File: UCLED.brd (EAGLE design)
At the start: 100 x 20 mm, 35 parts, among them CON1 CON-4P-TABS-JST_GH-RA, CON2 CON-4P-TABS-JST_GH-RA, CON3 PINHEAD_1X06-2, IC1 TJA1051, IC2 STM32F042F4PX, IC3 AP2127-3.3, J1 CONNECTION, J2 CONNECTION

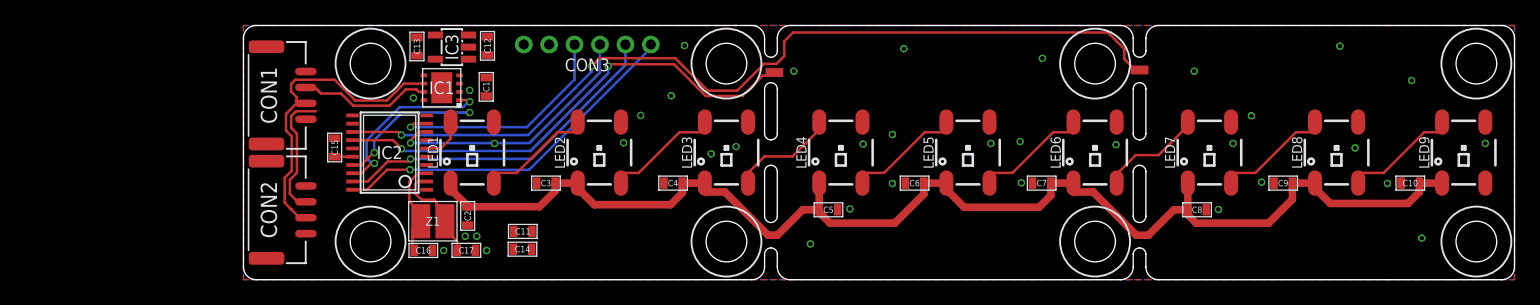
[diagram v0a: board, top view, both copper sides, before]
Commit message: V0.1 completed
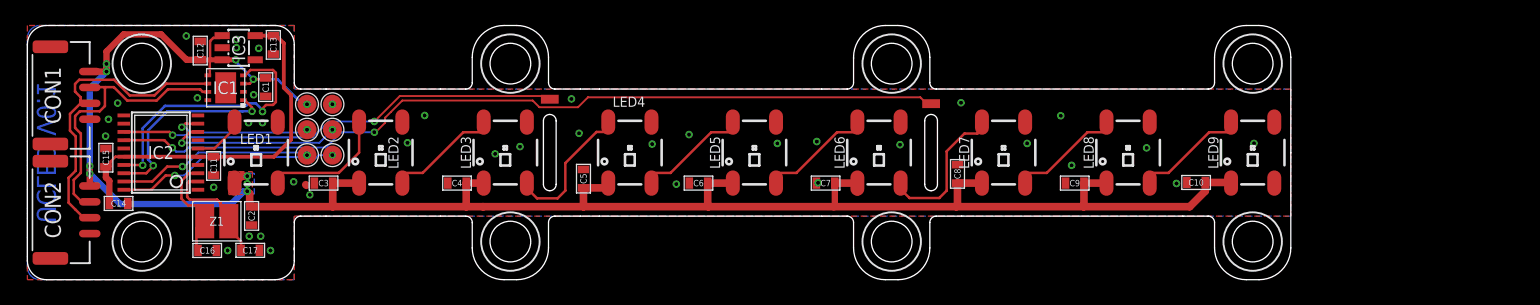
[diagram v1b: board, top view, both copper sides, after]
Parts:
- removed CON3: PINHEAD_1X06-2, pinhead:1X06-PTH-2
- added PAD1, PAD2, PAD3, PAD4, PAD5, PAD6: PAD-S_2X2, PADS:2х2
- added U$2: (no value), logo:DRAGON-30X13
- added U$3: (no value), logo:ZUBAX_20X9
- moved J2 46.5 mm to (23.1, 4.20)
- moved C14 32.0 mm to (-10.8, -4.00)
- moved C11 24.9 mm to (-3.35, -1.05), turned to 90 degrees
- moved C12 22.6 mm to (-4.40, 8.03), turned to 270 degrees
- moved C5 19.4 mm to (25.8, -2.05), turned to 270 degrees
- moved C8 19.1 mm to (55.2, -1.68), turned to 270 degrees
- moved C15 18.0 mm to (-11.8, -0.40)
- moved IC2 18.0 mm to (-7.50, 0.00)
- moved C3 17.5 mm to (5.30, -2.40)
- moved LED3 17.4 mm to (19.6, 0.00)
- moved C1 17.4 mm to (0.75, 5.15)
- moved LED2 17.2 mm to (9.80, 0.00)
- moved C16 17.0 mm to (-3.85, -7.70)
- moved C17 17.0 mm to (-0.47, -7.69)
- moved C2 17.0 mm to (-0.36, -4.98)
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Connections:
- net GND: now also PAD2.P$1; no longer CON3.5
- net SWCLK: now also PAD6.P$1; no longer CON3.1
- net SWDIO: now also PAD5.P$1; no longer CON3.2
- net USART2_RX: now also PAD3.P$1; no longer CON3.4
- net USART2_TX: now also PAD4.P$1; no longer CON3.3
- net VDD_5V: now also PAD1.P$1; no longer CON3.6
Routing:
- net VDD_5V: track 102.0 -> 161.5 mm, vias 0 -> 10
- net N$12: track 69.8 -> 34.8 mm
- net N$11: track 38.2 -> 66.2 mm
- net VDD_3V3: track 1.41 -> 29.0 mm
- net SWDIO: track 26.9 -> 15.4 mm, vias 1 -> 2
- net SWCLK: track 28.4 -> 17.9 mm, vias 1 -> 2
- net CAN_RX: track 11.5 -> 21.6 mm
- net USART2_TX: track 21.2 -> 14.1 mm, vias 1 -> 2
- net USART2_RX: track 18.6 -> 11.5 mm, vias 1 -> 2
- net N$8: track 8.17 -> 11.8 mm
- net N$4: track 8.41 -> 11.2 mm
- net N$23: track 21.0 -> 22.4 mm
- net N$35: track 26.1 -> 24.9 mm
- net CAN_TX: track 14.4 -> 15.6 mm
- net N$19: track 8.16 -> 9.18 mm
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- added copper zone on layer 1, net VDD_5V
- added copper zone on layer 16, net VDD_5V
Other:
- board size 100 x 20 mm -> 99.4 x 20 mm
- board text added: "UCLED V0.1"
